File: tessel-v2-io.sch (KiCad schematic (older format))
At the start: 65 parts

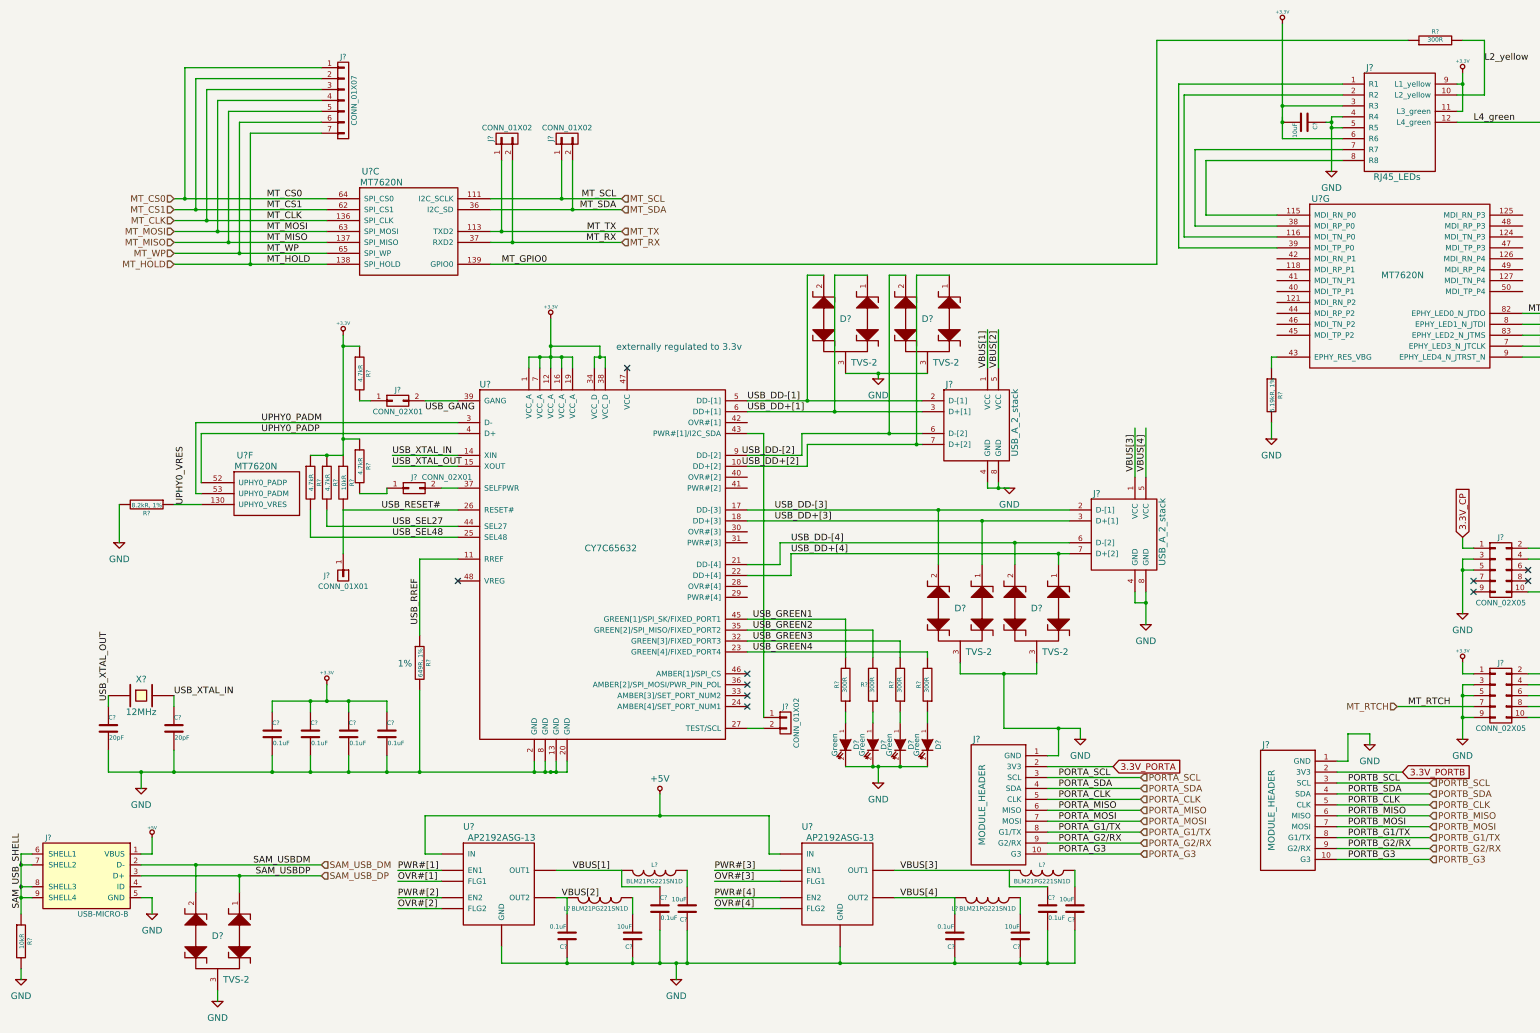
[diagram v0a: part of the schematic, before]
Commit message: labeling final nets
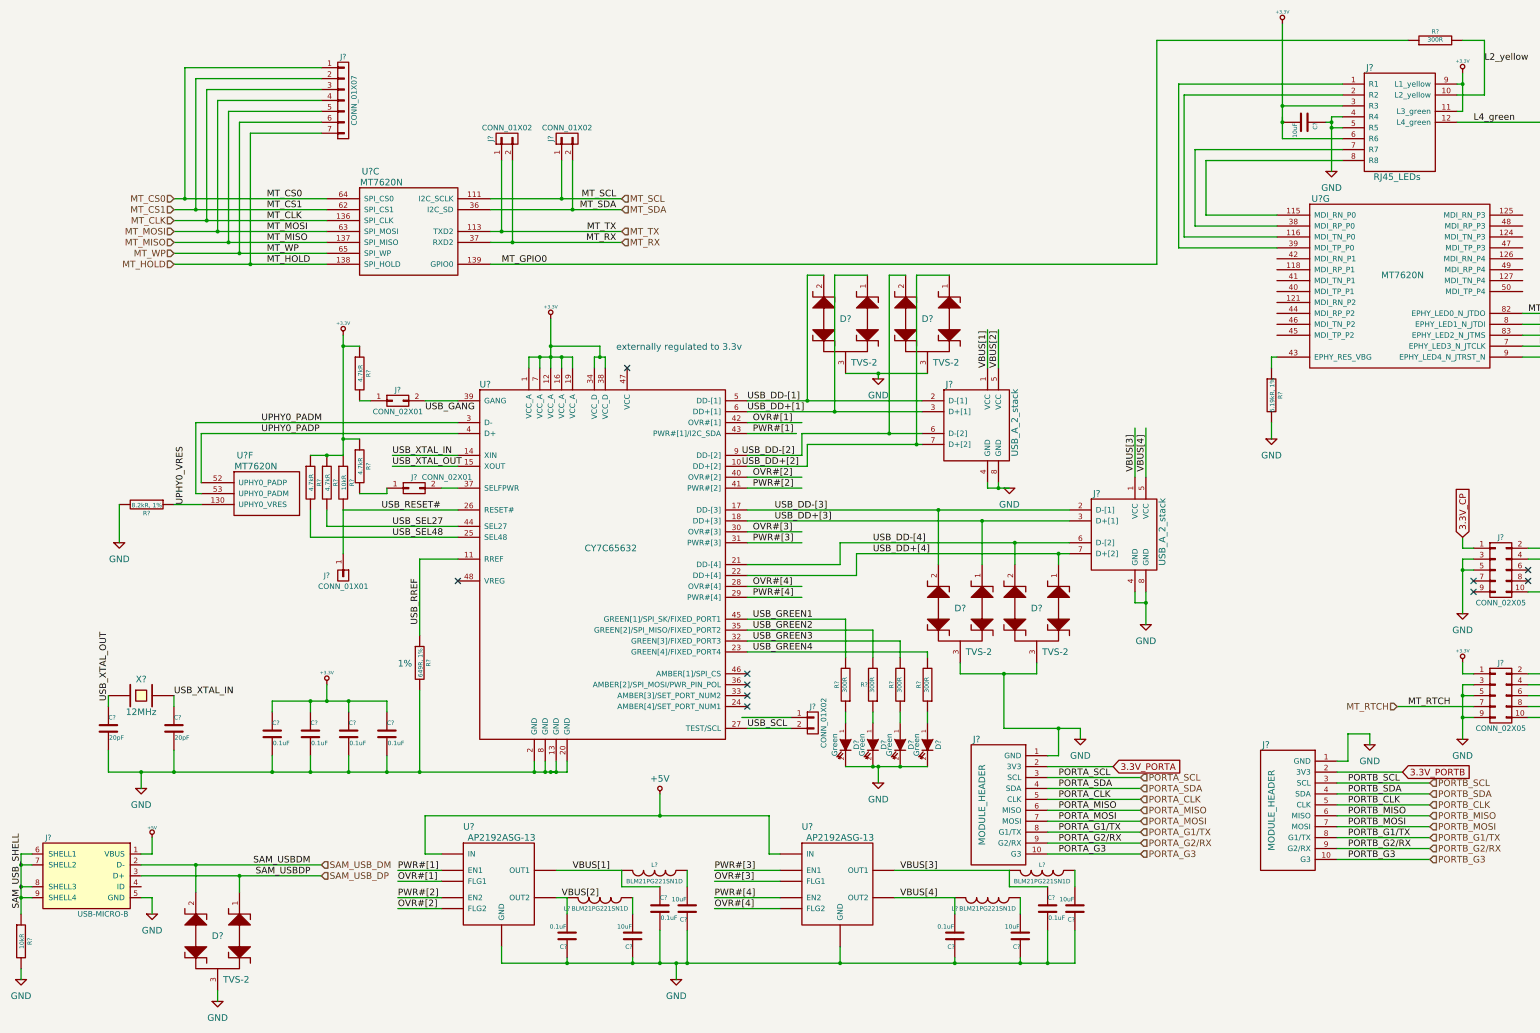
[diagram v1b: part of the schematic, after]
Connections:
- net labels added: USB_SCL
- wire segments 290 -> 369
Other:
- moved on the sheet: J?
